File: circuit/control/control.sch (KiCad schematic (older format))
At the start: 29 parts

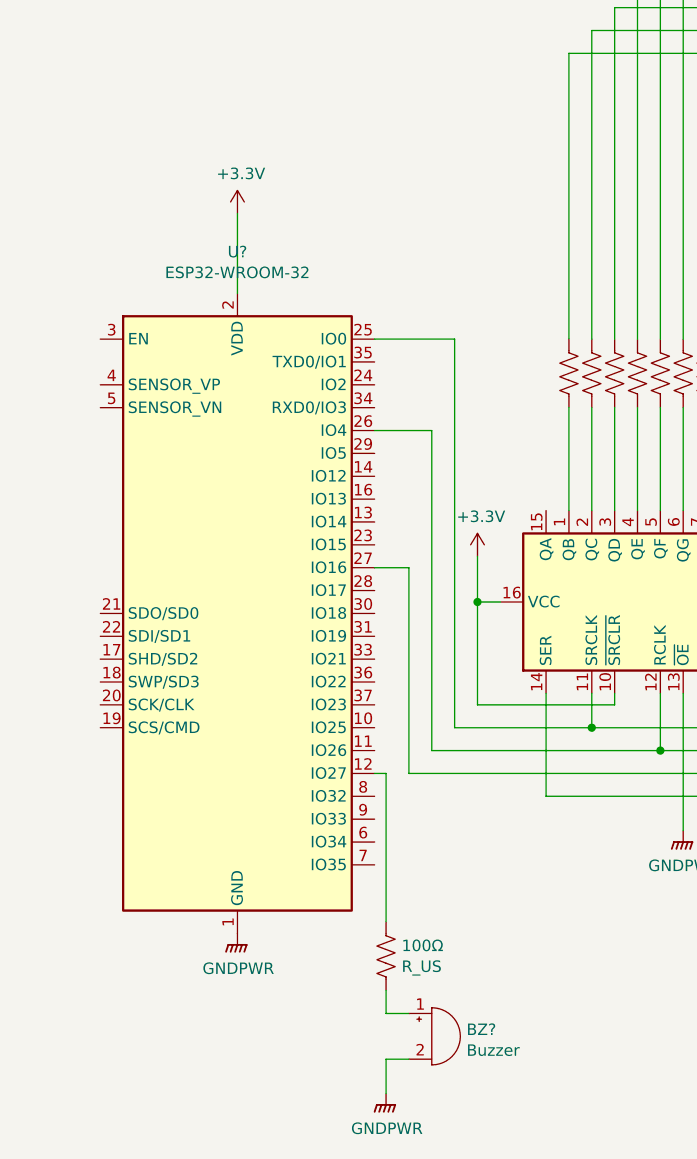
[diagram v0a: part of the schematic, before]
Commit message: [update] update circuit diagram
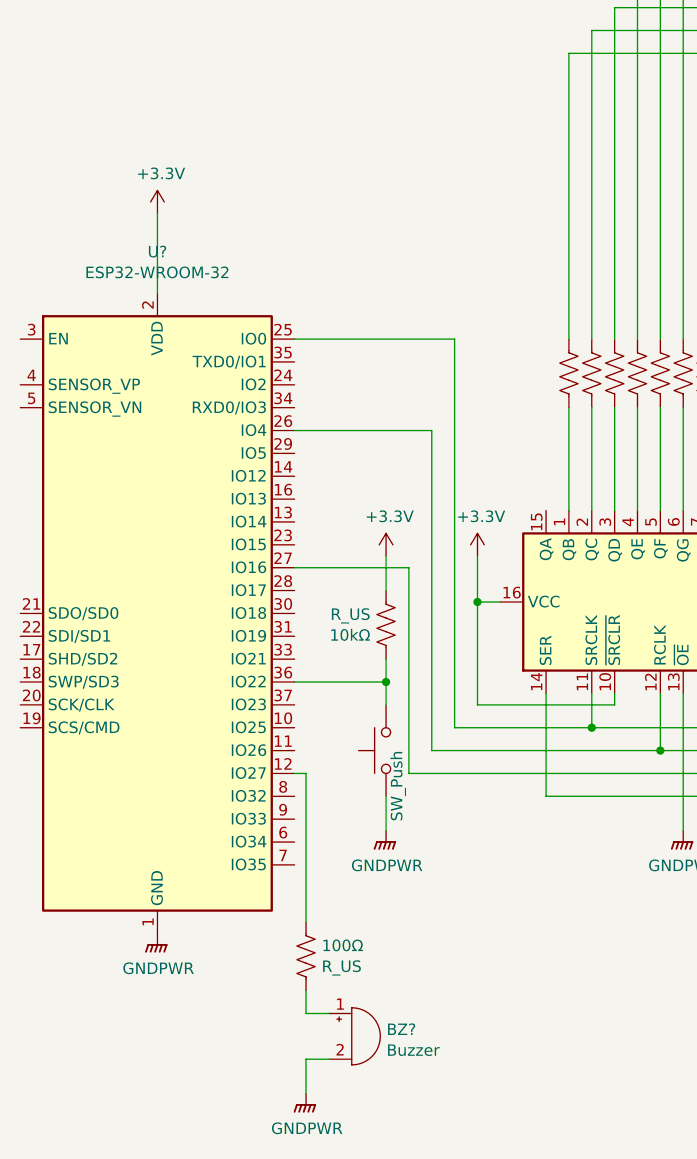
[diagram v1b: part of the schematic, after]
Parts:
- added 10kΩ: R_US, symbol Device:R_US
- added SW?: SW_Push, symbol Switch:SW_Push
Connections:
- net +3V3: now also 10kΩ.2
- net GNDPWR: now also SW?.1
- net at U?.36 (IO22): now also 10kΩ.1, SW?.2
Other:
- moved on the sheet: 100Ω, BZ?, U?
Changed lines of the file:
@@
 L RF_Module:ESP32-WROOM-32 U?
 U 1 1 6124F0F7
-P 2650 4300
-F 0 "U?" H 2650 5881 50  0000 C CNN
-F 1 "ESP32-WROOM-32" H 2650 5790 50  0000 C CNN
-F 2 "RF_Module:ESP32-WROOM-32" H 2650 2800 50  0001 C CNN
-F 3 "https://www.espressif.com/sites/default/files/documentation/esp32-wroom-32_datasheet_en.pdf" H 2350 4350 50  0001 C CNN
-	1    2650 4300
+P 2300 4300
+F 0 "U?" H 2300 5881 50  0000 C CNN
+F 1 "ESP32-WROOM-32" H 2300 5790 50  0000 C CNN
+F 2 "RF_Module:ESP32-WROOM-32" H 2300 2800 50  0001 C CNN
+F 3 "https://www.espressif.com/sites/default/files/documentation/esp32-wroom-32_datasheet_en.pdf" H 2000 4350 50  0001 C CNN
+	1    2300 4300
 	1    0    0    -1
 $EndComp
@@
 L power:GNDPWR #PWR?
 U 1 1 612CC9A8
-P 2650 5700
-F 0 "#PWR?" H 2650 5500 50  0001 C CNN
-F 1 "GNDPWR" H 2654 5546 50  0000 C CNN
-F 2 "" H 2650 5650 50  0001 C CNN
-F 3 "" H 2650 5650 50  0001 C CNN
-	1    2650 5700
+P 2300 5700
+F 0 "#PWR?" H 2300 5500 50  0001 C CNN
+F 1 "GNDPWR" H 2304 5546 50  0000 C CNN
+F 2 "" H 2300 5650 50  0001 C CNN
+F 3 "" H 2300 5650 50  0001 C CNN
+	1    2300 5700
 	1    0    0    -1
 $EndComp
@@
 L power:+3.3V #PWR?
 U 1 1 6174534F
-P 2650 2550
-F 0 "#PWR?" H 2650 2400 50  0001 C CNN
-F 1 "+3.3V" H 2665 2723 50  0000 C CNN
-F 2 "" H 2650 2550 50  0001 C CNN
-F 3 "" H 2650 2550 50  0001 C CNN
-	1    2650 2550
-	1    0    0    -1
-$EndComp
-Wire Wire Line
-	2650 2550 2650 2900
+P 2300 2550
+F 0 "#PWR?" H 2300 2400 50  0001 C CNN
+F 1 "+3.3V" H 2315 2723 50  0000 C CNN
+F 2 "" H 2300 2550 50  0001 C CNN
+F 3 "" H 2300 2550 50  0001 C CNN
+	1    2300 2550
+	1    0    0    -1
+$EndComp
+Wire Wire Line
+	2300 2550 2300 2900
 $Comp
 L Device:R_US 270Ω?
@@
 	1    0    0    -1
 $EndComp
-$Comp
-L Device:R_US 270Ω?
-U 1 1 61287533
-P 6750 3600
-F 0 "270Ω?" H 6818 3646 50  0001 L CNN
-F 1 "R_US" H 6818 3555 50  0001 L CNN
-F 2 "" V 6790 3590 50  0001 C CNN
-F 3 "~" H 6750 3600 50  0001 C CNN
-	1    6750 3600
-	1    0    0    -1
-$EndComp
 Wire Wire Line
 	6750 3450 6750 2150
@@
 $EndComp
 Wire Wire Line
-	3250 3100 3600 3100
-Wire Wire Line
-	3250 4100 3400 4100
-Wire Wire Line
-	3300 6050 3300 5950
+	2950 6050 2950 5950
 $Comp
 L Device:R_US 100Ω
 U 1 1 617204BC
-P 3300 5800
-F 0 "100Ω" H 3368 5846 50  0000 L CNN
-F 1 "R_US" H 3368 5755 50  0000 L CNN
-F 2 "" V 3340 5790 50  0001 C CNN
-F 3 "~" H 3300 5800 50  0001 C CNN
-	1    3300 5800
+P 2950 5800
+F 0 "100Ω" H 3018 5846 50  0000 L CNN
+F 1 "R_US" H 3018 5755 50  0000 L CNN
+F 2 "" V 2990 5790 50  0001 C CNN
+F 3 "~" H 2950 5800 50  0001 C CNN
+	1    2950 5800
 	1    0    0    -1
 $EndComp
@@
 L power:GNDPWR #PWR?
 U 1 1 612D5902
-P 3300 6400
-F 0 "#PWR?" H 3300 6200 50  0001 C CNN
-F 1 "GNDPWR" H 3304 6246 50  0000 C CNN
-F 2 "" H 3300 6350 50  0001 C CNN
-F 3 "" H 3300 6350 50  0001 C CNN
-	1    3300 6400
-	1    0    0    -1
-$EndComp
-Wire Wire Line
-	3300 6250 3300 6400
-Wire Wire Line
-	3400 6250 3300 6250
-Wire Wire Line
-	3300 6050 3400 6050
+P 2950 6400
+F 0 "#PWR?" H 2950 6200 50  0001 C CNN
+F 1 "GNDPWR" H 2954 6246 50  0000 C CNN
+F 2 "" H 2950 6350 50  0001 C CNN
+F 3 "" H 2950 6350 50  0001 C CNN
+	1    2950 6400
+	1    0    0    -1
+$EndComp
+Wire Wire Line
+	2950 6250 2950 6400
+Wire Wire Line
+	3050 6250 2950 6250
+Wire Wire Line
+	2950 6050 3050 6050
 $Comp
 L Device:Buzzer BZ?
 U 1 1 6126BBFF
-P 3500 6150
-F 0 "BZ?" H 3652 6179 50  0000 L CNN
-F 1 "Buzzer" H 3652 6088 50  0000 L CNN
-F 2 "" V 3475 6250 50  0001 C CNN
-F 3 "~" V 3475 6250 50  0001 C CNN
-	1    3500 6150
-	1    0    0    -1
-$EndComp
-Wire Wire Line
-	3250 3500 3500 3500
+P 3150 6150
+F 0 "BZ?" H 3302 6179 50  0000 L CNN
+F 1 "Buzzer" H 3302 6088 50  0000 L CNN
+F 2 "" V 3125 6250 50  0001 C CNN
+F 3 "~" V 3125 6250 50  0001 C CNN
+	1    3150 6150
+	1    0    0    -1
+$EndComp
 Wire Wire Line
 	3600 4800 4200 4800
@@
 	3400 4100 3400 5000
 Wire Wire Line
-	3250 5000 3300 5000
-Wire Wire Line
-	3300 5000 3300 5650
+	2900 5000 2950 5000
+Wire Wire Line
+	2950 5000 2950 5650
+Wire Wire Line
+	2900 3100 3600 3100
+Wire Wire Line
+	2900 3500 3500 3500
+Wire Wire Line
+	2900 4100 3400 4100
+Wire Wire Line
+	2900 4600 3300 4600
+$Comp
+L power:GNDPWR #PWR?
+U 1 1 616229BF
+P 3300 5250
+F 0 "#PWR?" H 3300 5050 50  0001 C CNN
+F 1 "GNDPWR" H 3304 5096 50  0000 C CNN
+F 2 "" H 3300 5200 50  0001 C CNN
+F 3 "" H 3300 5200 50  0001 C CNN
+	1    3300 5250
+	1    0    0    -1
+$EndComp
+$Comp
+L Device:R_US 270Ω?
+U 1 1 61287533
+P 6750 3600
+F 0 "270Ω?" H 6818 3646 50  0001 L CNN
+F 1 "R_US" H 6818 3555 50  0001 L CNN
+F 2 "" V 6790 3590 50  0001 C CNN
+F 3 "~" H 6750 3600 50  0001 C CNN
+	1    6750 3600
+	1    0    0    -1
+$EndComp
+Wire Wire Line
+	3300 4600 3300 4500
+$Comp
+L power:+3.3V #PWR?
+U 1 1 6165DB78
+P 3300 4050
+F 0 "#PWR?" H 3300 3900 50  0001 C CNN
+F 1 "+3.3V" H 3315 4223 50  0000 C CNN
+F 2 "" H 3300 4050 50  0001 C CNN
+F 3 "" H 3300 4050 50  0001 C CNN
+	1    3300 4050
+	1    0    0    -1
+$EndComp
+Wire Wire Line
+	3300 4050 3300 4200
+$Comp
+L Device:R_US 10kΩ
+U 1 1 6165705D
+P 3300 4350
+F 0 "10kΩ" H 3368 4396 50  0000 L CNN
+F 1 "R_US" H 3368 4305 50  0000 L CNN
+F 2 "" V 3340 4340 50  0001 C CNN
+F 3 "~" H 3300 4350 50  0001 C CNN
+	1    3300 4350
+	-1   0    0    1
+$EndComp
+Wire Wire Line
+	3300 4600 3300 4700
+Connection ~ 3300 4600
+Wire Wire Line
+	3300 5100 3300 5250
+$Comp
+L Switch:SW_Push SW?
+U 1 1 616981A3
+P 3300 4900
+F 0 "SW?" H 3300 5185 50  0001 C CNN
+F 1 "SW_Push" H 3300 4852 50  0000 R CNN
+F 2 "" H 3300 5100 50  0001 C CNN
+F 3 "~" H 3300 5100 50  0001 C CNN
+	1    3300 4900
+	0    -1   -1   0
+$EndComp
 $EndSCHEMATC
